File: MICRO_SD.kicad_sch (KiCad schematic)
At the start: 10 parts, among them J12 10067099-200LF

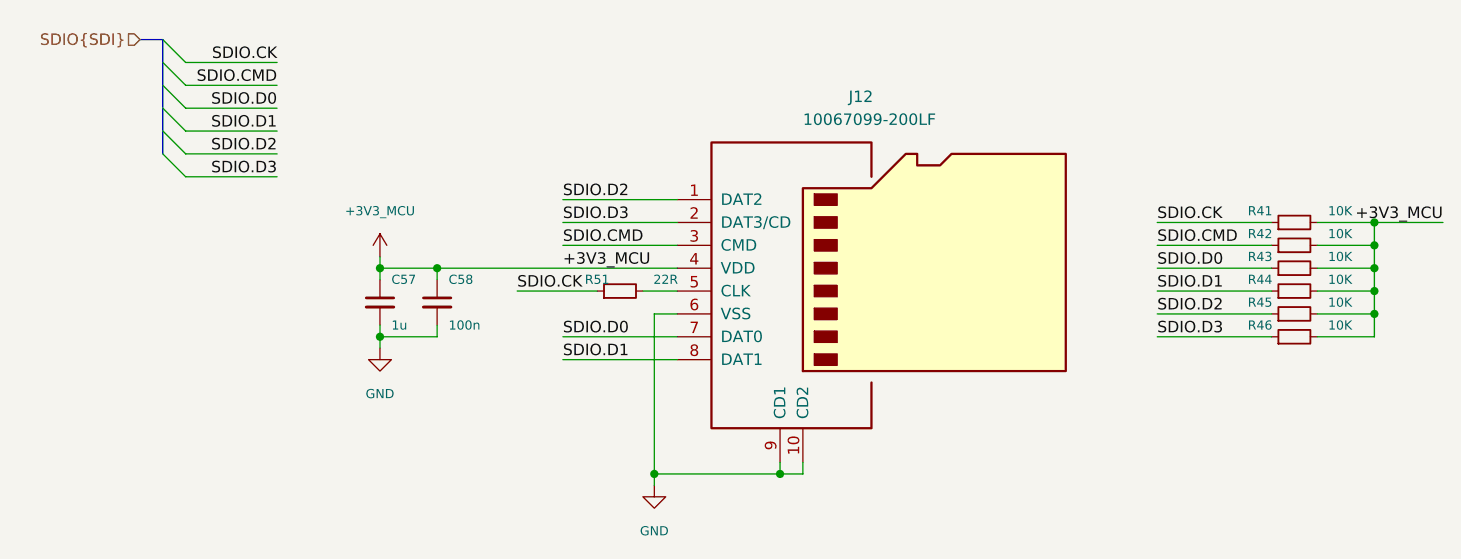
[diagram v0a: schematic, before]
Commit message: pos down
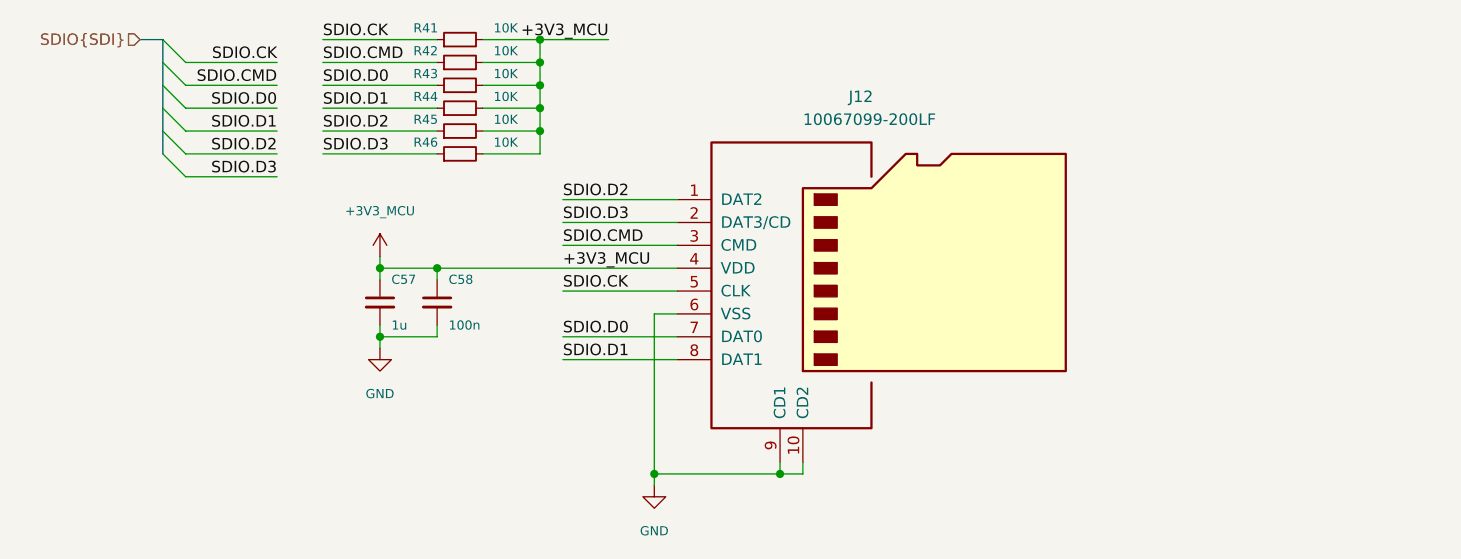
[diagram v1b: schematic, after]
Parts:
- removed R51: 22R, Resistor_SMD:R_0402_1005Metric, symbol FC01_Project:MICRO_SD__R_Small
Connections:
- net SDIO.CK: now also J12.5 (CLK)
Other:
- moved on the sheet: R41, R42, R43, R44, R45, R46
